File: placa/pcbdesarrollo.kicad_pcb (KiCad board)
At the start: 2 copper layers, 81.7 x 107.1 mm, 57 parts, among them J1 DB9, K1 I2C, P1 CONN_3X2, P2 BATT, P3 CONN_3, SW1 PULSADOR, SW2 RESET, U1 MAX232, U2 AVR_ATMEGA88, U3 7805FIX, U4 7133, X1 18.432 Mhz

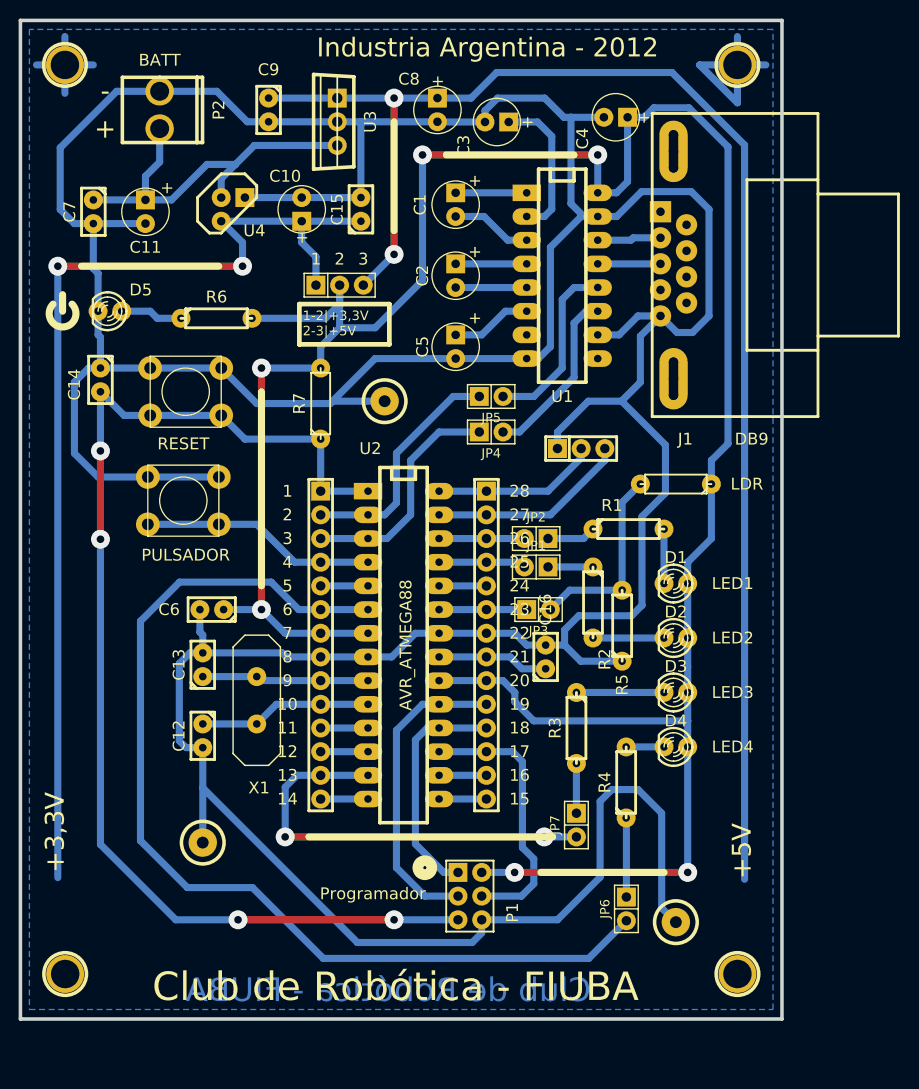
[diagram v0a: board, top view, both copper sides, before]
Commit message: version 2 del pcb
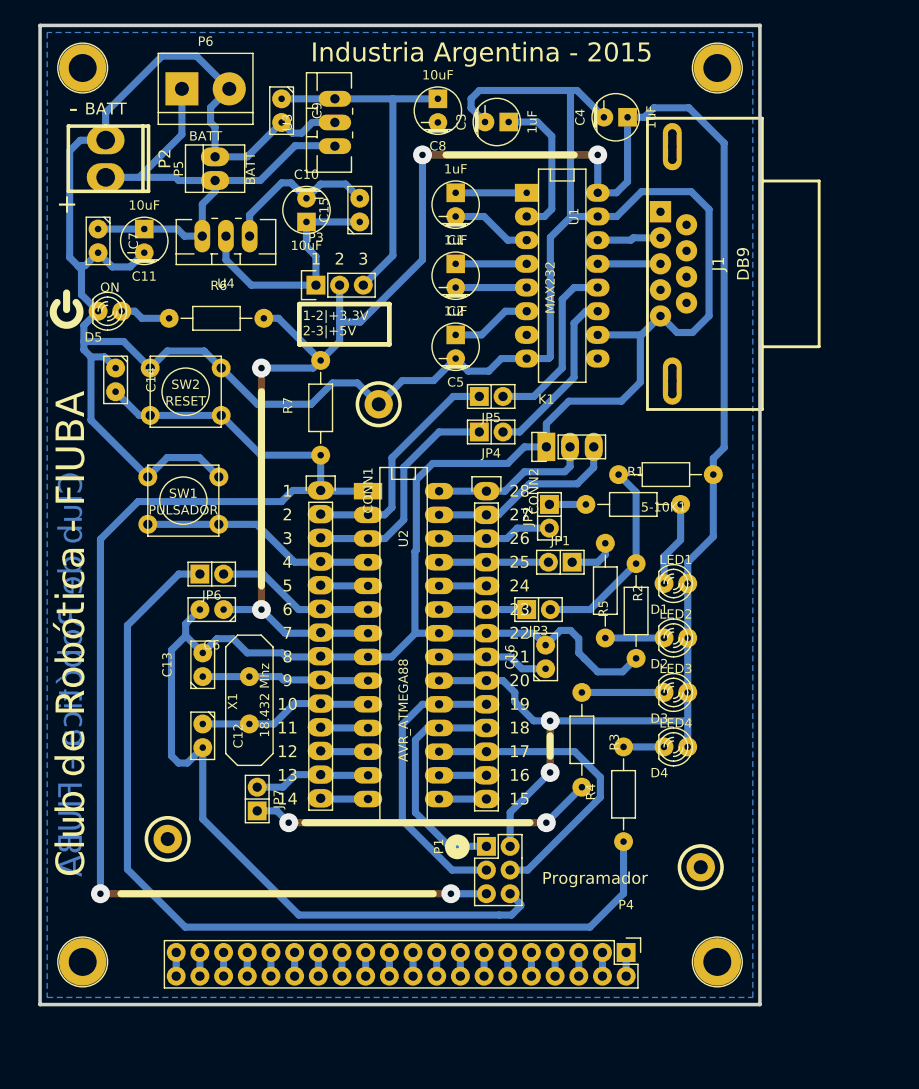
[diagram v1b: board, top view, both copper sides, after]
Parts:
- removed the 1PIN at (135.3, 78.5)
- removed the 1PIN at (173.1, 140.0)
- removed the 1PIN at (101.0, 42.5)
- removed the 1PIN at (173.1, 42.5)
- added 1PIN: P***, 1pin, F.Cu at (134.6, 78.9)
- added 1PIN: P***, 1pin, F.Cu at (102.9, 42.8)
- added 1PIN: P***, 1pin, F.Cu at (170.9, 138.7)
- added 1PIN: P***, 1pin, F.Cu at (170.9, 42.8)
- added P4: CONN_02X20, Socket_Strips:Socket_Strip_Straight_2x20, F.Cu at (161.2, 137.7)
- added P5: BATT, Connect:PINHEAD1-2, F.Cu at (117.1, 53.6)
- added P6: BATT, Connect:bornier2, F.Cu at (116.1, 45.0)
- 5-10K1, R1, R2, R3, R4, R5, R6, R7: footprint R3 -> Resistors_ThroughHole:Resistor_Horizontal_RM10mm
- C1, C10, C11, C2, C3, C4, C5, C8: footprint C1V5 -> Capacitors_ThroughHole:Capacitor5x6RM2.5
- C12, C13, C14, C15, C16, C6, C7, C9: footprint C1 -> Capacitors_ThroughHole:Capacitor3MMDiscRM2.5
- CONN1, CONN2: footprint SIL-14 -> Socket_Strips:Socket_Strip_Straight_1x14
- D1, D2, D3, D4, D5: footprint LED-3MM -> LEDs:LED-3MM
- J1: footprint DB9H -> Popurri_CDR:DB9-F
- K1: footprint SIL-3 -> Socket_Strips:Socket_Strip_Straight_1x03
- P1: footprint pin_array_3x2 -> Socket_Strips:Socket_Strip_Straight_2x03
- P2: footprint molex_2_recto -> Popurri_CDR:molex_2_recto
- P3: footprint PIN_ARRAY_3X1 -> Socket_Strips:Socket_Strip_Straight_1x03
- SW1, SW2: footprint SW_PUSH_SMALL -> Discret:SW_PUSH_SMALL
- U1: footprint DIP-16__300_ELL -> Sockets_DIP:DIP-16__300_ELL
- U2: footprint DIP-28__300_ELL -> Sockets_DIP:DIP-28__300_ELL
- U3: footprint TO220V-123 -> Transistors_TO-220:TO-220_Neutral123_Vertical_LargePads
- U4: value 7133 -> AP1117T33; footprint TO92 -> Transistors_TO-220:TO-220_Neutral123_Vertical_LargePads
- X1: footprint HC-18UV -> Discret:HC-18UV
- moved JP6 57.2 mm to (116.7, 97.1), turned to 180 degrees
- moved JP7 34.4 mm to (121.6, 121.2), turned to 270 degrees
- moved CONN1 16.6 mm to (128.4, 88.1)
- moved CONN2 16.5 mm to (146.2, 88.2)
- moved P2 7.80 mm to (105.3, 52.5)
- moved 1PIN 6.47 mm to (169.2, 128.5)
- moved P1 5.62 mm to (146.2, 126.3), turned to 90 degrees
- moved 1PIN 3.78 mm to (112.0, 125.5)
- moved K1 3.74 mm to (152.6, 83.4)
- moved C7 3.17 mm to (104.5, 61.3)
- moved C11 3.13 mm to (109.5, 61.3), turned to 180 degrees
- moved U4 2.97 mm to (118.2, 60.8), turned to 180 degrees
- moved JP2 2.78 mm to (152.9, 90.9), turned to 90 degrees
- moved R1 2.69 mm to (161.9, 89.6)
- moved JP1 2.64 mm to (154.1, 95.8)
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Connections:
- U4 pad 2: VDD -> +3.3V
- U4 pad 3: +3.3V -> VDD
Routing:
- net +5V: track 155.6 -> 38.1 mm, vias 2 -> 0
- net /LED4: track 109.9 -> 17.1 mm
- net Net-(JP6-Pad1): track 8.53 -> 99.1 mm
- net +3.3V: track 113.6 -> 26.2 mm, vias 2 -> 0
- net GND: track 520.7 -> 461.1 mm
- net /LED3: track 46.0 -> 12.4 mm, vias 2 -> 0
- net Net-(JP7-Pad1): track 5.33 -> 36.9 mm, vias 0 -> 2
- net VCC: track 272.7 -> 245.7 mm
- net VDD: track 41.1 -> 55.8 mm
- net /RESET: track 126.7 -> 138.9 mm, vias 4 -> 2
- net /MOSI: track 29.1 -> 33.5 mm
- net Net-(D1-Pad2): track 5.84 -> 9.22 mm
- net /LED1: track 9.14 -> 12.3 mm
- net /CC20: track 0.00 -> 2.54 mm
- net /CC19: track 0.00 -> 2.54 mm
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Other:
- board size 81.7 x 107.1 mm -> 77.2 x 105 mm
- net class Default: via_drill 0.8128 -> 0.7
- board text added: "Industria Argentina - 2015"
- board text removed: "+3,3V"
- board text removed: "+5V"
- board text removed: "Industria Argentina - 2012"

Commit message: version 2 del pcb
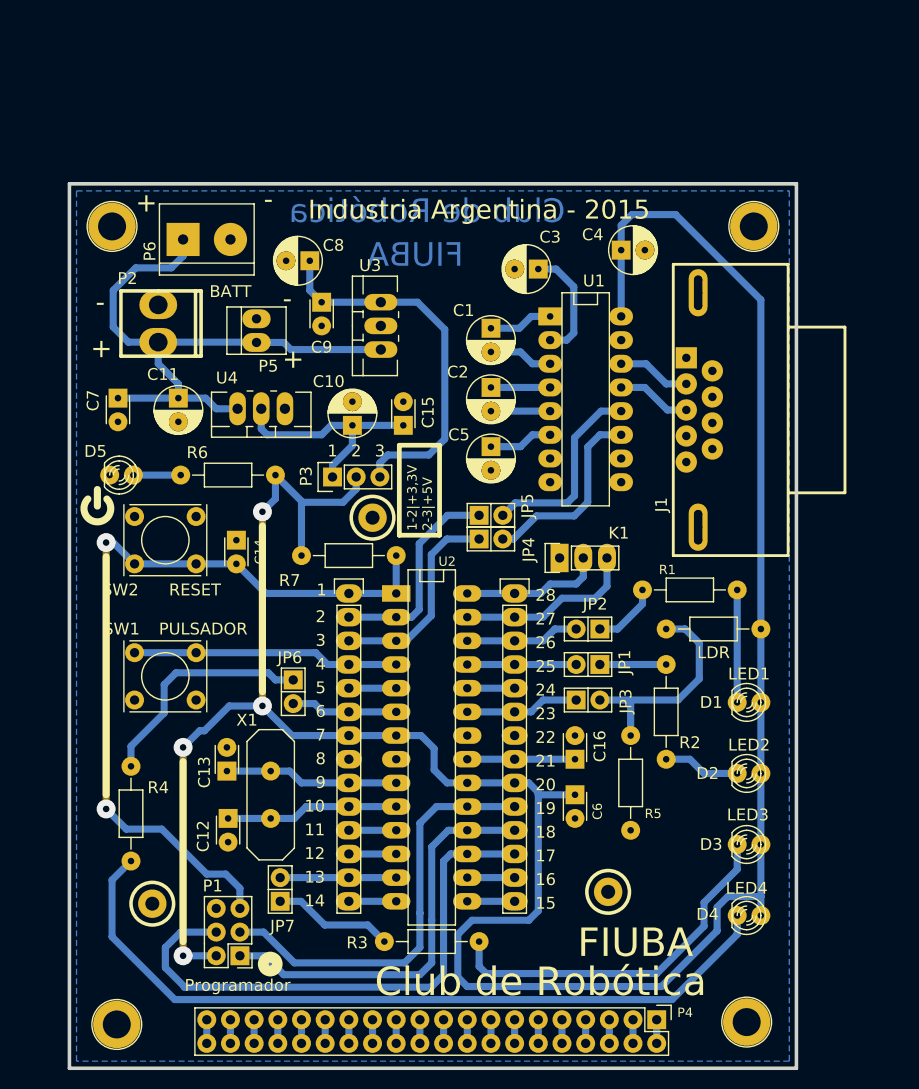
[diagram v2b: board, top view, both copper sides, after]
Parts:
- removed 5-10K1: LDR, Resistors_ThroughHole:Resistor_Horizontal_RM10mm
- added LDR: LDR 5-10 k, Resistors_ThroughHole:Resistor_Horizontal_RM10mm, F.Cu at (170.5, 103.0)
- C1, C10, C11, C2, C3, C4, C5, C8: footprint Capacitors_ThroughHole:Capacitor5x6RM2.5 -> Popurri_CDR:C_Radial_D5_L6_P2.5
- C12, C13, C14, C15, C16, C6, C7, C9: footprint Capacitors_ThroughHole:Capacitor3MMDiscRM2.5 -> Capacitors_ThroughHole:C_Disc_D3_P2.5
- moved R4 52.9 mm to (108.1, 122.8), turned to 270 degrees
- moved C6 43.7 mm to (155.7, 120.8), turned to 270 degrees
- moved P1 28.9 mm to (119.7, 138.0), turned to 270 degrees
- moved R3 27.0 mm to (140.3, 136.5), turned to 180 degrees
- moved C10 23.6 mm to (131.8, 81.1), turned to 90 degrees
- moved C15 23.6 mm to (137.3, 81.1)
- moved U3 22.4 mm to (134.8, 70.5)
- moved C14 21.5 mm to (119.4, 93.4)
- moved C8 21.2 mm to (127.2, 63.5)
- moved C9 21.0 mm to (128.5, 67.9)
- moved P3 20.7 mm to (129.7, 86.7)
- moved D4 19.7 mm to (174.3, 133.7)
- moved SW1 18.9 mm to (111.7, 108.1), turned to 180 degrees
- moved U4 18.9 mm to (122.0, 79.3)
- moved P2 18.6 mm to (111.0, 70.2)
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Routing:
- net GND: track 461.1 -> 0.00 mm
- net Net-(D4-Pad2): track 4.34 -> 84.0 mm
- net Net-(JP6-Pad1): track 99.1 -> 24.9 mm
- net /RESET: track 138.9 -> 86.4 mm
- net VCC: track 245.7 -> 279.0 mm, vias 6 -> 4
- net Net-(D3-Pad2): track 8.81 -> 39.5 mm
- net /MOSI: track 33.5 -> 59.9 mm
- net Net-(JP7-Pad1): track 36.9 -> 13.0 mm, vias 2 -> 0
- net /MISO: track 25.1 -> 44.0 mm
- net /SCK: track 31.4 -> 45.6 mm
- net VDD: track 55.8 -> 64.6 mm
- net /LED4: track 17.1 -> 11.4 mm
- net Net-(C3-Pad1): track 16.1 -> 12.4 mm
- net Net-(JP2-Pad1): track 3.91 -> 7.20 mm
- net /BOTON: track 25.3 -> 28.6 mm
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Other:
- board size 77.2 x 105 mm -> 78 x 94.9 mm
- rule trace_min: 0.0254 -> 0.3048
- rule via_min_size: 0.889 -> 2.032
- board text added: "Club de Robótica"
- board text added: "FIUBA"
- board text removed: "Club de Robótica - FIUBA"

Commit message: actualizacion de la placa
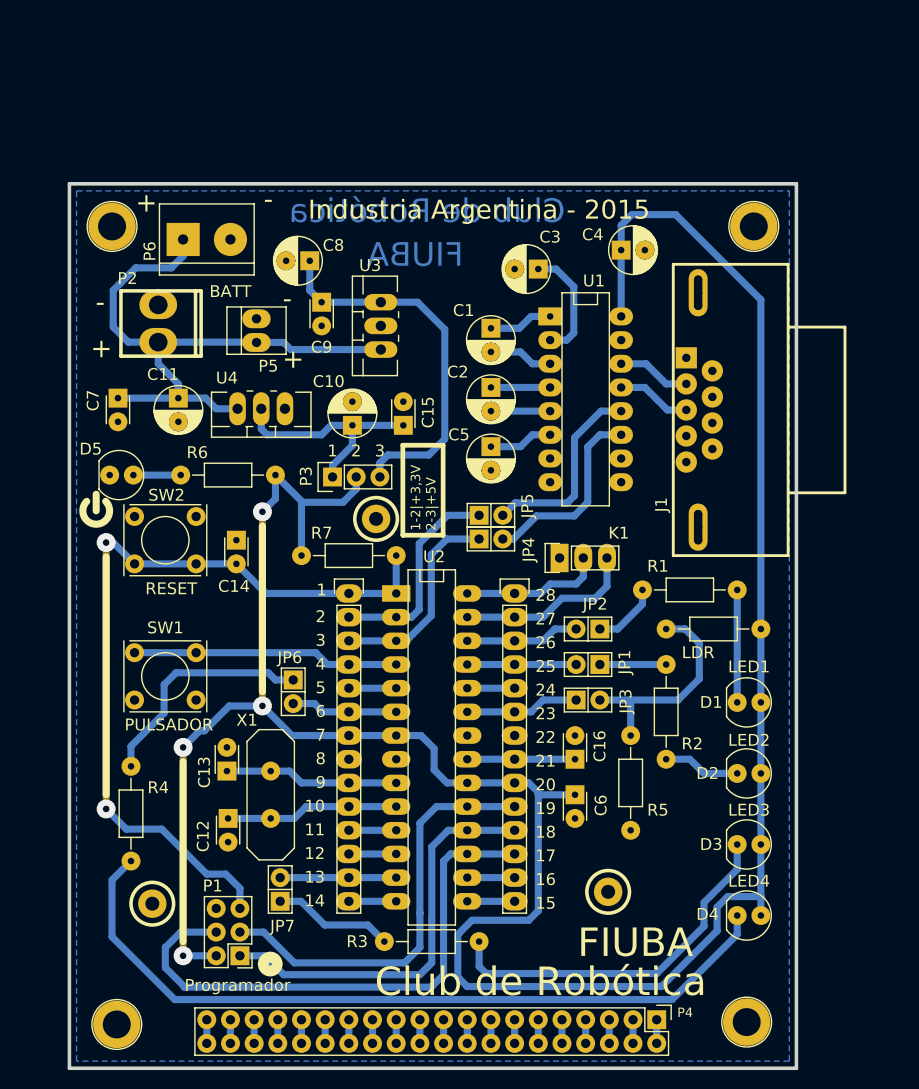
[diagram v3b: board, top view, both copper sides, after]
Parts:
- moved 1PIN 0.40 mm to (134.3, 91.2)
